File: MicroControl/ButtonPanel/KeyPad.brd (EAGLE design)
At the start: 66.3 x 110.2 mm, 15 parts

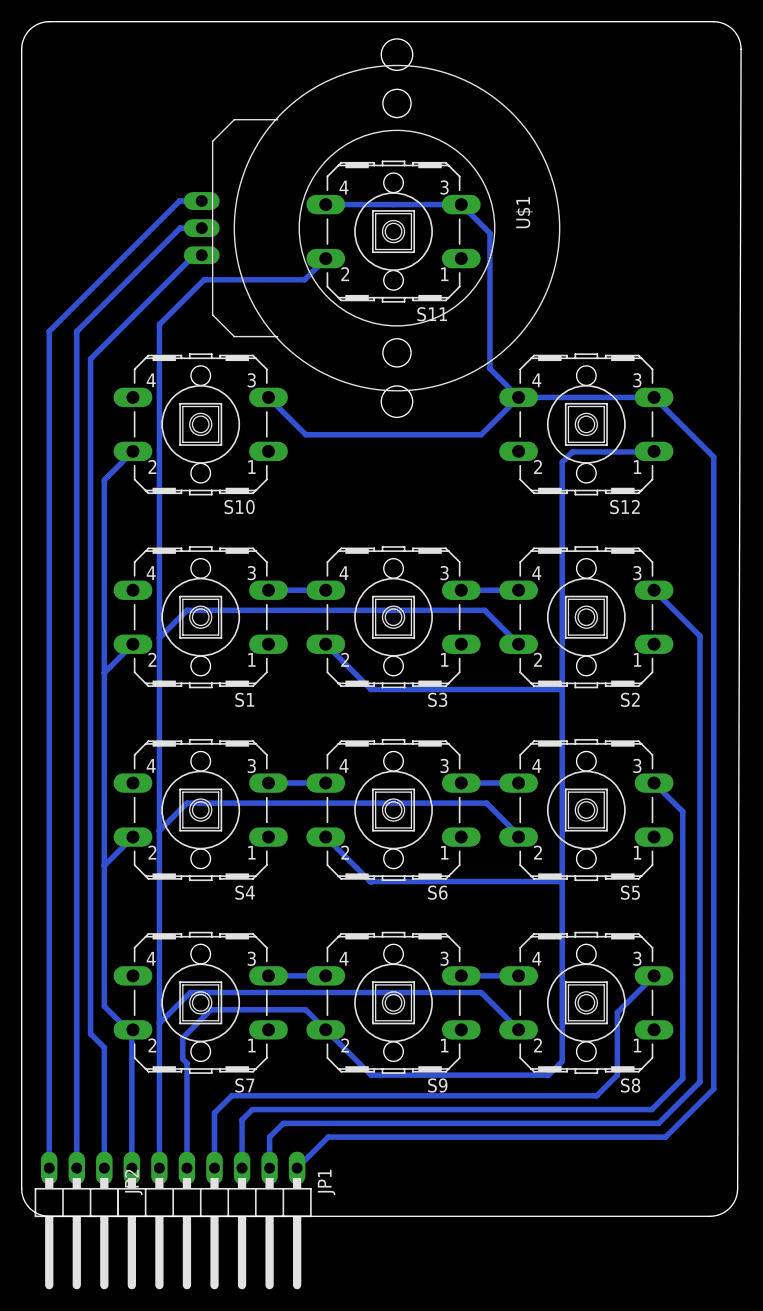
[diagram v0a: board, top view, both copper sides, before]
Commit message: more accurate
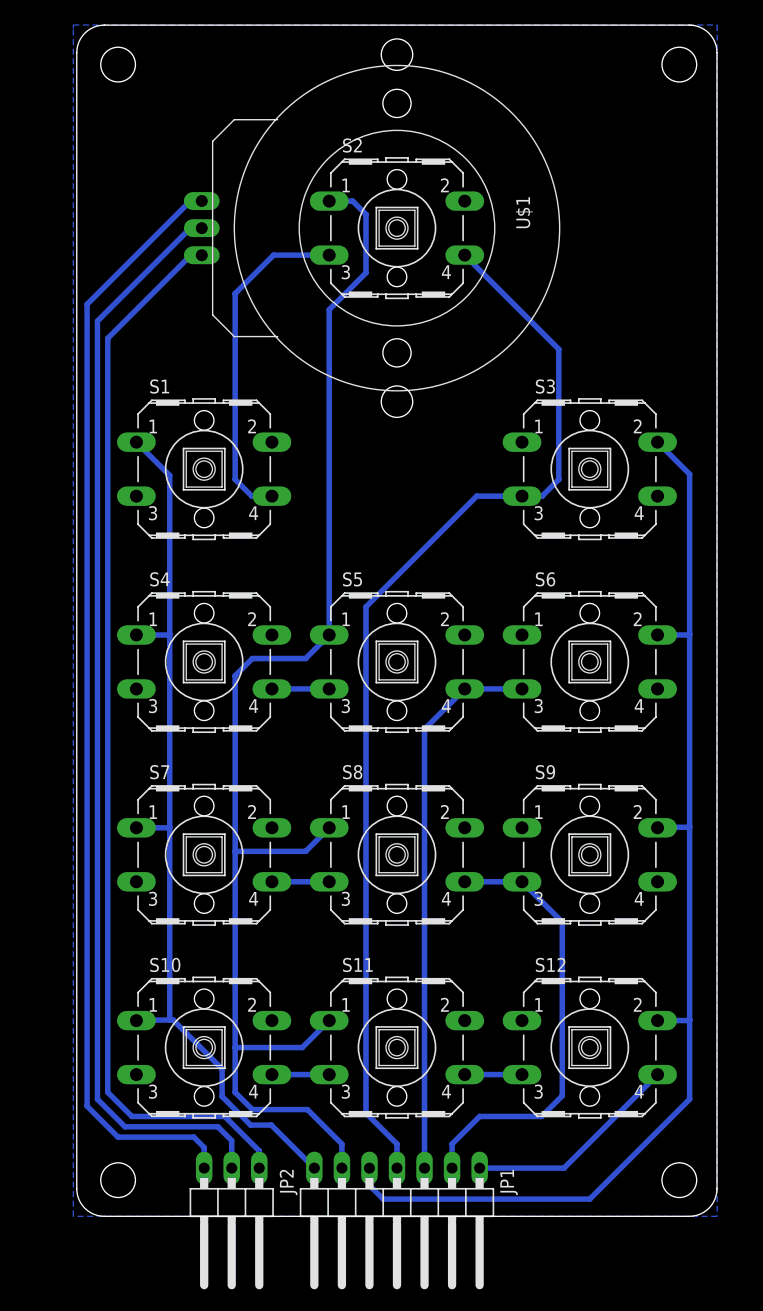
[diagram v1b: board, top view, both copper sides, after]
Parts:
- moved S11 75.2 mm to (29.5, 16.2), turned to 0 degrees
- moved S10 57.5 mm to (11.7, 16.2), turned to 0 degrees
- moved S12 57.5 mm to (47.3, 16.2), turned to 0 degrees
- moved S2 39.9 mm to (29.5, 91.8), turned to 0 degrees
- moved S3 22.7 mm to (47.3, 69.5), turned to 0 degrees
- moved S6 22.7 mm to (47.3, 51.8), turned to 0 degrees
- moved S9 22.7 mm to (47.3, 34.0), turned to 0 degrees
- moved S5 22.2 mm to (29.5, 51.8), turned to 0 degrees
- moved S8 22.2 mm to (29.5, 34.0), turned to 0 degrees
- moved JP1 16.8 mm to (29.5, 1.27)
- moved JP2 14.3 mm to (14.3, 1.27)
- moved S1 13.7 mm to (11.7, 69.5), turned to 0 degrees
- moved S4 13.7 mm to (11.7, 51.8), turned to 0 degrees
- moved S7 13.7 mm to (11.7, 34.0), turned to 0 degrees
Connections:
- removed net N$16: S1.3, S3.4
- net N$10: now also S1.4, S2.3; no longer JP1.6, S11.2, S2.2, S5.2, S8.2
- net N$11: now also JP1.4, S2.4, S3.3; no longer S7.3, S9.4
- net N$12: now also JP1.1, S12.4; no longer S5.4, S6.3
- net N$13: now also JP1.7, S1.1, S10.1, S4.1, S7.1; no longer JP1.5, S12.1, S3.2, S6.2, S9.2
- net N$14: now also JP1.6, S11.1, S2.1, S5.1, S8.1; no longer S4.3, S6.4
- net N$15: now also JP1.5, S12.2, S3.2, S6.2, S9.2; no longer S2.4, S3.3
- net N$4: now also S10.4, S11.3; no longer JP1.2, S2.3
- net N$5: now also S11.4, S12.3; no longer JP1.3, S5.3
- net N$6: now also JP1.2, S8.4, S9.3; no longer JP1.4, S8.3
- net N$7: now also S7.4, S8.3; no longer JP1.1, S10.3, S11.3, S11.4, S12.3, S12.4
- net N$8: now also S4.4, S5.3; no longer JP1.7, S1.2, S10.2, S4.2, S7.2
- net N$9: now also JP1.3, S5.4, S6.3; no longer S8.4, S9.3
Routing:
- net N$7: track 178.4 -> 5.28 mm
- net N$10: track 202.4 -> 31.3 mm
- net N$14: track 5.28 -> 126.1 mm
- net N$15: track 5.28 -> 106.2 mm
- net N$11: track 5.28 -> 99.9 mm
- net N$4: track 91.8 -> 5.28 mm
- net N$13: track 162.6 -> 84.3 mm
- net N$8: track 76.0 -> 5.28 mm
- net N$5: track 75.0 -> 5.28 mm
- net N$9: track 5.28 -> 51.0 mm
- net N$12: track 5.28 -> 20.0 mm
- net N$6: track 54.2 -> 40.8 mm
- net N$2: track 89.4 -> 99.2 mm
- net N$1: track 92.6 -> 101.4 mm
- net N$3: track 96.2 -> 102.7 mm
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- added copper zone on layer 16, net N$16
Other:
- board size 66.3 x 110.2 mm -> 59 x 109.8 mm
